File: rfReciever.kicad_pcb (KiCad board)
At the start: 2 copper layers, 82 x 40 mm, 27 parts, among them P1 USB_C_Plug_USB2.0, SW1 SW_Push, SW2 SW_Push, U1 XBee_SMT, U2 CP2102N-Axx-xQFN20, U3 USBLC6-2SC6

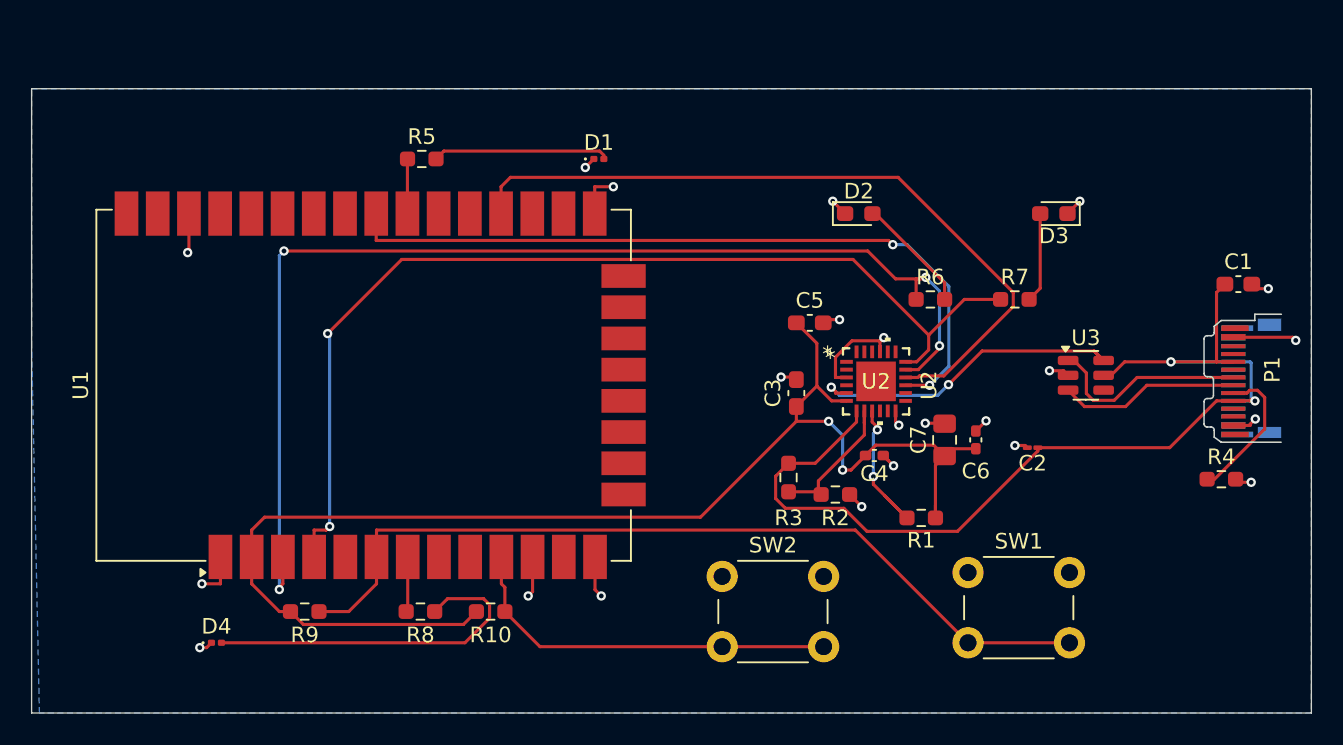
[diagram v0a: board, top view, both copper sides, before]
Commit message: Final Schematic preliminary pcb layout(pre-routing)
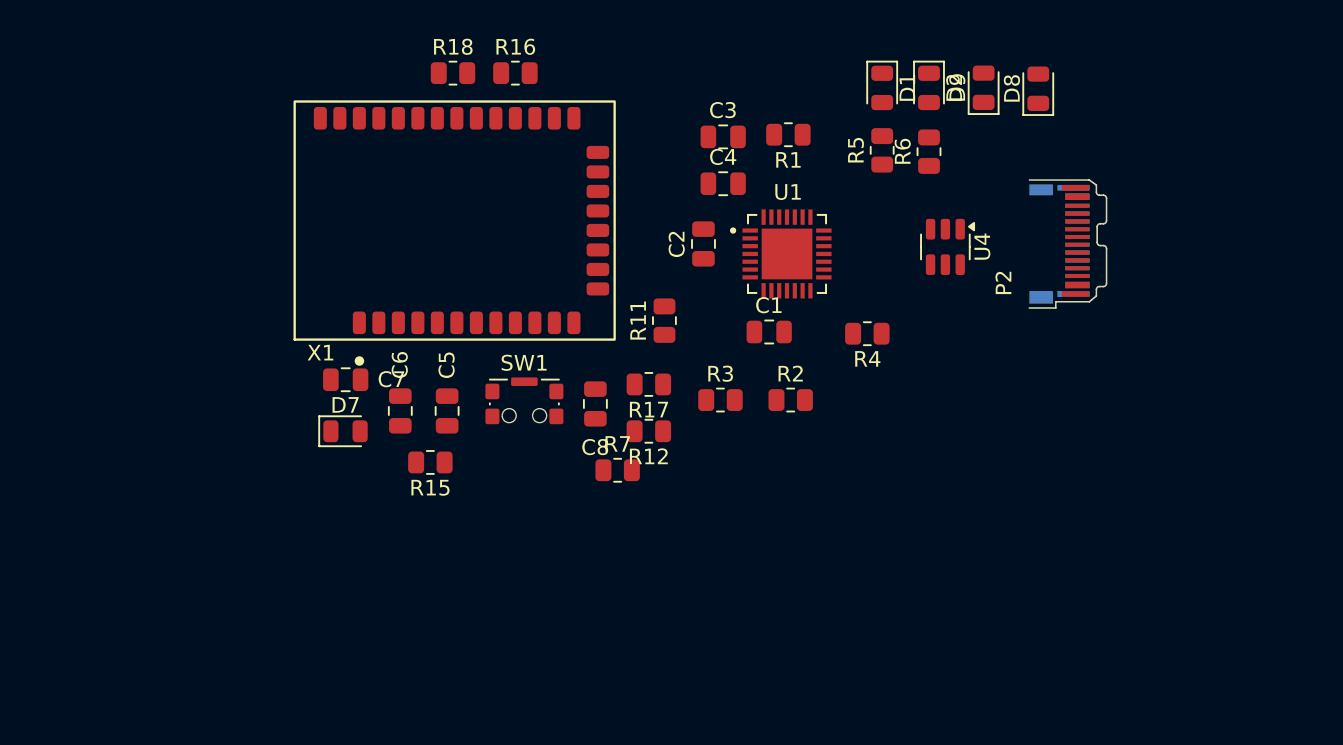
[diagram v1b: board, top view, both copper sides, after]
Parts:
- removed D3: LED, LED_SMD:LED_0603_1608Metric_Pad1.05x0.95mm_HandSolder
- removed D4: LED, LED_SMD:LED_0201_0603Metric
- removed P1: USB_C_Plug_USB2.0, Connector_USB:USB_C_Plug_JAE_DX07P024AJ1
- removed R10, R9: 10k, Resistor_SMD:R_0603_1608Metric_Pad0.98x0.95mm_HandSolder
- removed R8: 330, Resistor_SMD:R_0603_1608Metric_Pad0.98x0.95mm_HandSolder
- removed SW2: SW_Push, Button_Switch_THT:SW_PUSH_6mm_H4.3mm
- removed U2: CP2102N-Axx-xQFN20, Audio_Module:QFN24_CP2102N_SIL
- removed U3: USBLC6-2SC6, Package_TO_SOT_SMD:SOT-23-6
- added C8: 1u, Capacitor_SMD:C_0805_2012Metric, F.Cu at (93.6, 82.2)
- added D7: LED, LED_SMD:LED_0805_2012Metric, F.Cu at (77.6, 83.9)
- added D8: LED, LED_SMD:LED_0805_2012Metric, F.Cu at (122.0, 62.0)
- added D9: LED, LED_SMD:LED_0805_2012Metric, F.Cu at (118.5, 61.9)
- added P2: USB_C_Plug_USB2.0, Connector_USB:USB_C_Plug_JAE_DX07P024AJ1, F.Cu at (123.4, 71.8)
- added R11: 10K, Resistor_SMD:R_0805_2012Metric, F.Cu at (98.1, 76.9)
- added R12: 10k, Resistor_SMD:R_0805_2012Metric, F.Cu at (97.1, 83.9)
- added R15: 1K, Resistor_SMD:R_0805_2012Metric, F.Cu at (83.1, 85.9)
- added R16: 1K, Resistor_SMD:R_0805_2012Metric, F.Cu at (88.5, 61.0)
- added R17: 10k, Resistor_SMD:R_0805_2012Metric, F.Cu at (97.1, 80.9)
- added R18: 1K, Resistor_SMD:R_0805_2012Metric, F.Cu at (84.5, 61.0)
- added U4: USBLC6-2SC6, Package_TO_SOT_SMD:SOT-23-6, F.Cu at (116.0, 72.1)
- added X1: DigiXBeeRX900Micro, rfReciever-Footprints:XBeeXR900RFMicro, F.Cu at (85.1, 70.4)
- C1, C3: footprint Capacitor_SMD:C_0603_1608Metric_Pad1.08x0.95mm_HandSolder -> Capacitor_SMD:C_0805_2012Metric
- C2: footprint Capacitor_SMD:C_01005_0402Metric_Pad0.57x0.30mm_HandSolder -> Capacitor_SMD:C_0805_2012Metric
- C4: footprint Capacitor_SMD:C_0402_1005Metric_Pad0.74x0.62mm_HandSolder -> Capacitor_SMD:C_0805_2012Metric
- C5: value 1uF -> 47pF; footprint Capacitor_SMD:C_0603_1608Metric_Pad1.08x0.95mm_HandSolder -> Capacitor_SMD:C_0805_2012Metric
- C6: value 47pF -> 1uF; footprint Capacitor_SMD:C_0402_1005Metric_Pad0.74x0.62mm_HandSolder -> Capacitor_SMD:C_0805_2012Metric
- C7: footprint Capacitor_SMD:C_0805_2012Metric_Pad1.18x1.45mm_HandSolder -> Capacitor_SMD:C_0805_2012Metric
- D1: footprint LED_SMD:LED_0201_0603Metric -> LED_SMD:LED_0805_2012Metric
- D2: footprint LED_SMD:LED_0603_1608Metric_Pad1.05x0.95mm_HandSolder -> LED_SMD:LED_0805_2012Metric
- R1, R2, R3, R4: footprint Resistor_SMD:R_0603_1608Metric_Pad0.98x0.95mm_HandSolder -> Resistor_SMD:R_0805_2012Metric
- R5: value 330 -> 1K; footprint Resistor_SMD:R_0603_1608Metric_Pad0.98x0.95mm_HandSolder -> Resistor_SMD:R_0805_2012Metric
- R6: value 220 -> 1K; footprint Resistor_SMD:R_0603_1608Metric_Pad0.98x0.95mm_HandSolder -> Resistor_SMD:R_0805_2012Metric
- R7: value 220 -> 1k; footprint Resistor_SMD:R_0603_1608Metric_Pad0.98x0.95mm_HandSolder -> Resistor_SMD:R_0805_2012Metric
- SW1: value SW_Push -> RF_RESET; footprint Button_Switch_THT:SW_PUSH_6mm_H4.3mm -> Button_Switch_SMD:SW_SPST_CK_KMS2xxGP
- U1: value XBee_SMT -> CP2102N-Axx-xQFN20; footprint RF_Module:Digi_XBee_SMT -> rfReciever-Footprints:QFN50P500X500X80-29N
- moved C7 38.6 mm to (77.6, 80.6), turned to 180 degrees
- moved C6 36.9 mm to (81.1, 82.6), turned to -90 degrees
- moved SW1 30.4 mm to (89.1, 82.2)
- moved C1 30.2 mm to (104.8, 77.6)
- moved R5 29.5 mm to (112.0, 65.9), turned to 90 degrees
- moved U1 27.7 mm to (105.9, 72.6), turned to 0 degrees
- moved R7 27.7 mm to (95.1, 86.4)
- moved R1 26.0 mm to (106.0, 64.9)
- moved C2 24.8 mm to (100.6, 71.9), turned to 90 degrees
- moved R4 24.5 mm to (111.1, 77.7), turned to 180 degrees
- moved C5 23.9 mm to (84.1, 82.6), turned to -90 degrees
- moved C4 19.9 mm to (101.8, 68.1), turned to 0 degrees
- moved D1 18.7 mm to (112.0, 61.9), turned to -90 degrees
- moved C3 17.1 mm to (101.8, 65.1), turned to 0 degrees
- moved R6 9.47 mm to (115.0, 66.0), turned to 90 degrees
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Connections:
- net Net-(D1-A) renamed /BRIDGE_D1
- net Net-(D2-A) renamed /BRIDGE_D2
- C1 pad 1: /5V(in) -> +5V
- C2 pad 1: /5V(in) -> +5V
- C3 pad 2: /3.3V (out) -> +3.3V
- C4 pad 2: /3.3V (out) -> +3.3V
- C5 pad 1: /3.3V (out) -> +3.3V
- C6 pad 1: /3.3V (out) -> +3.3V
- C7 pad 1: /3.3V (out) -> +3.3V
- R1 pad 1: /3.3V (out) -> /BRIDGE_3.3
- R1 pad 2: Net-(U2-~{RST}) -> +3.3V
- R2 pad 1: Net-(U2-VBUS) -> /BRIDGE_VBUS
- R3 pad 1: /5V(in) -> +5V
- R3 pad 2: Net-(U2-VBUS) -> /BRIDGE_VBUS
- R5 pad 1: Net-(U1-DIO5/ASSOCIATE) -> /TXD(Bridge)
- R6 pad 1: Net-(U1-DIO13/UART_TX) -> /RXD(Bridge)
- R7 pad 1: Net-(U1-DIO14/UART_RX/~{CONFIG}) -> /RF_RESET
- R7 pad 2: Net-(D3-A) -> /RF_RESET
- SW1 pad 1: GND -> /RF_RESET
- SW1 pad 2: Net-(U1-RESET/OD_OUT) -> GND
- U1 pad 1: GND -> unconnected-(U1-RS485/GPIO.1-Pad1)
- U1 pad 10: Net-(U1-DIO8/SLEEP_REQUEST) -> unconnected-(U1-NC-Pad10)
- U1 pad 11: GND -> unconnected-(U1-~{SUSPEND}-Pad11)
- U1 pad 12: unconnected-(U1-DIO19/SPI_~{ATTN}-Pad12) -> GND
- U1 pad 13: GND -> unconnected-(U1-~{WAKEUP}-Pad13)
- U1 pad 15: unconnected-(U1-DIO17/SPI_~{SSEL}-Pad15) -> /CTS(Bridge)
- U1 pad 16: unconnected-(U1-DIO16/SPI_MOSI-Pad16) -> /RTS(Bridge)
- U1 pad 17: unconnected-(U1-DIO15/SPI_MISO-Pad17) -> /RXD(Bridge)
- U1 pad 18: unconnected-(U1-NC-Pad18) -> /TXD(Bridge)
- U1 pad 2: /3.3V (out) -> unconnected-(U1-CLK/GPIO.0-Pad2)
- U1 pad 21: unconnected-(U1-NC-Pad21) -> GND
- U1 pad 22: GND -> (no net)
- U1 pad 23: unconnected-(U1-NC-Pad23) -> (no net)
- U1 pad 24: unconnected-(U1-DIO4-Pad24) -> (no net)
- U1 pad 25: Net-(U1-DIO7/~{CTS}) -> (no net)
- U1 pad 26: unconnected-(U1-DIO9/ON/~{SLEEP}-Pad26) -> (no net)
- U1 pad 27: unconnected-(U1-VREF-Pad27) -> (no net)
- U1 pad 28: Net-(U1-DIO5/ASSOCIATE) -> (no net)
- U1 pad 29: Net-(U1-DIO6/~{RTS}) -> (no net)
- U1 pad 3: Net-(U1-DIO13/UART_TX) -> GND
- U1 pad 4: Net-(U1-DIO14/UART_RX/~{CONFIG}) -> /USB_D+
- U1 pad 5: unconnected-(U1-DIO12-Pad5) -> /USB_D-
- U1 pad 6: Net-(U1-RESET/OD_OUT) -> +3.3V
- U1 pad 7: Net-(U1-DIO10/RSSI/PWM0) -> +5V
- U1 pad 8: unconnected-(U1-DIO11/PWM1-Pad8) -> /BRIDGE_VBUS
- U1 pad 9: unconnected-(U1-NC-Pad9) -> /BRIDGE_3.3
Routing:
- net /3.3V (out): track 87.0 -> 0.00 mm, vias 2 -> 0
- net Net-(U1-DIO13/UART_TX): track 74.9 -> 0.00 mm, vias 4 -> 0
- net /5V(in): track 67.7 -> 0.00 mm, vias 2 -> 0
- net Net-(U1-DIO14/UART_RX/~{CONFIG}): track 66.0 -> 0.00 mm, vias 2 -> 0
- net Net-(U1-RESET/OD_OUT): track 55.3 -> 0.00 mm
- net Net-(U1-DIO6/~{RTS}): track 48.0 -> 0.00 mm, vias 2 -> 0
- net Net-(U1-DIO7/~{CTS}): track 47.5 -> 0.00 mm
- net GND: track 42.2 -> 0.00 mm, vias 23 -> 0
- net Net-(U1-DIO8/SLEEP_REQUEST): track 25.0 -> 0.00 mm
- net Net-(D4-A): track 22.7 -> 0.00 mm
- net Net-(U2-D-): track 21.2 -> 0.00 mm, vias 2 -> 0
- net /D-: track 13.0 -> 0.00 mm
- net /D+: track 11.6 -> 0.00 mm
- net /BRIDGE_D1: track 11.3 -> 0.00 mm
- net Net-(U2-~{RST}): track 10.3 -> 0.00 mm, vias 2 -> 0
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- removed copper zone on B.Cu, net GND
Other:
- board size 82 x 40 mm -> 5 x 8.2 mm
- board text removed: "U2"
